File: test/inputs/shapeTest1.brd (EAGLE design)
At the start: 2 parts

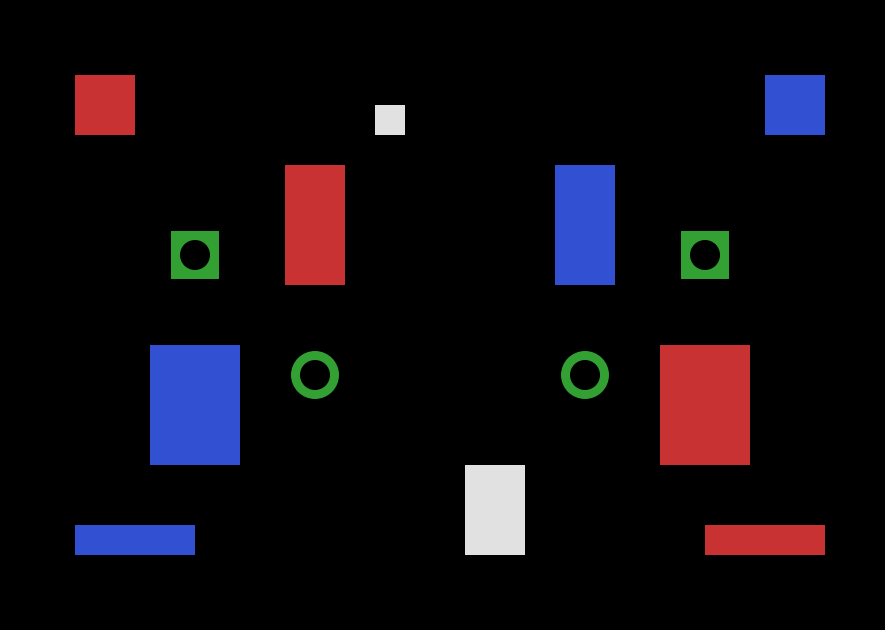
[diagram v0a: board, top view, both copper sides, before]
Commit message: Improved tests
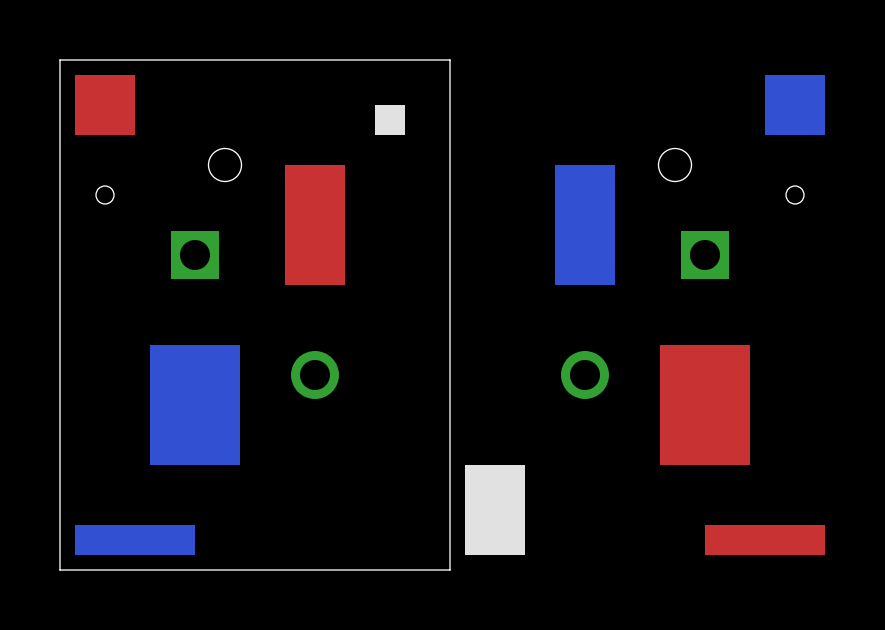
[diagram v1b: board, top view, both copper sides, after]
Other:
- board outline added: 13 x 17 mm
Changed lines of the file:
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@@
 <setting verticaltext="up"/>
 </settings>
-<grid distance="1" unitdist="mm" unit="mm" style="lines" multiple="1" display="yes" altdistance="0.025" altunitdist="inch" altunit="inch"/>
+<grid distance="0.5" unitdist="mm" unit="mm" style="lines" multiple="1" display="yes" altdistance="0.025" altunitdist="inch" altunit="inch"/>
 <layers>
 <layer number="1" name="Top" color="4" fill="1" visible="yes" active="yes"/>
@@
 <layer number="97" name="Info" color="7" fill="1" visible="no" active="no"/>
 <layer number="98" name="Guide" color="6" fill="1" visible="no" active="no"/>
-<layer number="101" name="tTest2" color="13" fill="1" visible="yes" active="yes"/>
-<layer number="102" name="bTest2" color="14" fill="1" visible="yes" active="yes"/>
+<layer number="102" name="onBoard" color="10" fill="3" visible="yes" active="yes"/>
+<layer number="103" name="offBoard" color="9" fill="3" visible="yes" active="yes"/>
+<layer number="151" name="tTest2" color="13" fill="1" visible="yes" active="yes"/>
+<layer number="152" name="bTest2" color="14" fill="1" visible="yes" active="yes"/>
 </layers>
 <board>
 <plain>
+<wire x1="-6.5" y1="8.5" x2="6.5" y2="8.5" width="0" layer="20"/>
+<wire x1="6.5" y1="8.5" x2="6.5" y2="-8.5" width="0" layer="20"/>
+<wire x1="6.5" y1="-8.5" x2="-6.5" y2="-8.5" width="0" layer="20"/>
+<wire x1="-6.5" y1="-8.5" x2="-6.5" y2="8.5" width="0" layer="20"/>
 </plain>
 <attributes>
